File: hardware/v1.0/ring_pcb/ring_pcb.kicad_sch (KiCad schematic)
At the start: 18 parts

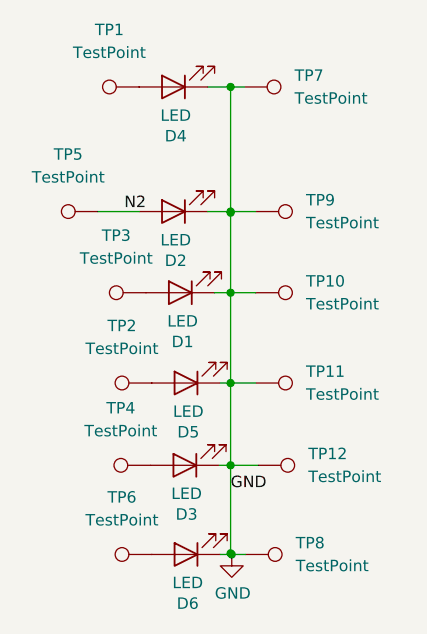
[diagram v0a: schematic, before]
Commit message: New PCB and Gerbers
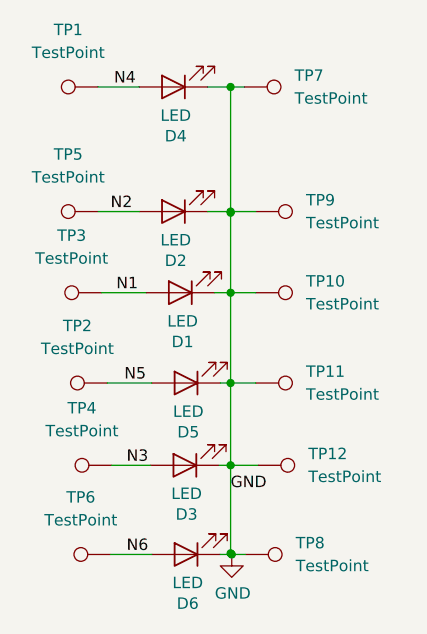
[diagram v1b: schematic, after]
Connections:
- net N4: now reaches D4.2 (A), TP1.1
- net N5: now reaches D5.2 (A), TP2.1
- net N3: now reaches D3.2 (A), TP4.1
- net N6: now reaches D6.2 (A), TP6.1
- net N1: now reaches D1.2 (A), TP3.1
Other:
- moved on the sheet: TP1, TP2, TP3, TP4, TP6
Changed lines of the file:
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@@
 (kicad_sch (version 20210621) (generator eeschema)
   (paper "A4")
+  (junction (at 127.508 87.757) (diameter 0) (color 0 0 0 0))
+  (junction (at 127.508 78.74) (diameter 0) (color 0 0 0 0))
   (junction (at 127.508 116.713) (diameter 0) (color 0 0 0 0))
-  (junction (at 127.508 87.757) (diameter 0) (color 0 0 0 0))
-  (junction (at 127.508 106.934) (diameter 0) (color 0 0 0 0))
-  (junction (at 127.508 78.74) (diameter 0) (color 0 0 0 0))
-  (junction (at 127.508 64.897) (diameter 0) (color 0 0 0 0))
   (junction (at 127.508 78.867) (diameter 0) (color 0 0 0 0))
   (junction (at 127.508 97.79) (diameter 0) (color 0 0 0 0))
+  (junction (at 127.508 64.897) (diameter 0) (color 0 0 0 0))
+  (junction (at 127.508 106.934) (diameter 0) (color 0 0 0 0))
   (junction (at 127.635 116.84) (diameter 0) (color 0 0 0 0))
+  (wire (pts (xy 113.792 97.79) (xy 118.745 97.79))
+    (stroke (width 0) (type default) (color 0 0 0 0))
+  )
   (wire (pts (xy 130.302 78.74) (xy 127.508 78.74))
     (stroke (width 0) (type default) (color 0 0 0 0))
@@
     (stroke (width 0) (type default) (color 0 0 0 0))
   )
+  (wire (pts (xy 114.173 116.84) (xy 118.745 116.84))
+    (stroke (width 0) (type default) (color 0 0 0 0))
+  )
   (wire (pts (xy 130.556 106.934) (xy 127.508 106.934))
     (stroke (width 0) (type default) (color 0 0 0 0))
   )
+  (wire (pts (xy 114.3 106.934) (xy 118.618 106.934))
+    (stroke (width 0) (type default) (color 0 0 0 0))
+  )
   (wire (pts (xy 112.776 78.74) (xy 117.348 78.74))
     (stroke (width 0) (type default) (color 0 0 0 0))
@@
     (stroke (width 0) (type default) (color 0 0 0 0))
   )
+  (wire (pts (xy 127.508 87.757) (xy 127.508 78.867))
+    (stroke (width 0) (type default) (color 0 0 0 0))
+  )
   (wire (pts (xy 127.508 78.867) (xy 127.508 78.74))
     (stroke (width 0) (type default) (color 0 0 0 0))
@@
     (stroke (width 0) (type default) (color 0 0 0 0))
   )
-  (wire (pts (xy 127.508 87.757) (xy 127.508 78.867))
+  (wire (pts (xy 127.508 97.79) (xy 127.508 87.757))
     (stroke (width 0) (type default) (color 0 0 0 0))
   )
@@
     (stroke (width 0) (type default) (color 0 0 0 0))
   )
-  (wire (pts (xy 127.508 97.79) (xy 127.508 87.757))
-    (stroke (width 0) (type default) (color 0 0 0 0))
-  )
   (wire (pts (xy 129.032 64.897) (xy 127.508 64.897))
     (stroke (width 0) (type default) (color 0 0 0 0))
@@
     (stroke (width 0) (type default) (color 0 0 0 0))
   )
+  (wire (pts (xy 112.776 64.897) (xy 117.348 64.897))
+    (stroke (width 0) (type default) (color 0 0 0 0))
+  )
+  (wire (pts (xy 129.159 116.84) (xy 127.635 116.84))
+    (stroke (width 0) (type default) (color 0 0 0 0))
+  )
   (wire (pts (xy 127.635 116.84) (xy 126.365 116.84))
     (stroke (width 0) (type default) (color 0 0 0 0))
   )
-  (wire (pts (xy 129.159 116.84) (xy 127.635 116.84))
-    (stroke (width 0) (type default) (color 0 0 0 0))
-  )
   (wire (pts (xy 126.238 106.934) (xy 127.508 106.934))
     (stroke (width 0) (type default) (color 0 0 0 0))
@@
     (stroke (width 0) (type default) (color 0 0 0 0))
   )
+  (wire (pts (xy 113.157 87.757) (xy 118.11 87.757))
+    (stroke (width 0) (type default) (color 0 0 0 0))
+  )
+  (label "N3" (at 115.951 106.934 0)
+    (effects (font (size 1.27 1.27)) (justify left bottom))
+  )
   (label "GND" (at 127.508 109.855 0)
     (effects (font (size 1.27 1.27)) (justify left bottom))
   )
-  (label "N2" (at 115.697 78.74 0)
+  (label "N1" (at 114.808 87.757 0)
+    (effects (font (size 1.27 1.27)) (justify left bottom))
+  )
+  (label "N5" (at 115.697 97.79 0)
+    (effects (font (size 1.27 1.27)) (justify left bottom))
+  )
+  (label "N2" (at 114.173 78.74 0)
+    (effects (font (size 1.27 1.27)) (justify left bottom))
+  )
+  (label "N4" (at 114.554 64.897 0)
+    (effects (font (size 1.27 1.27)) (justify left bottom))
+  )
+  (label "N6" (at 115.951 116.84 0)
     (effects (font (size 1.27 1.27)) (justify left bottom))
   )
@@
     (pin "2")
   )
-  (symbol (lib_id "Connector:TestPoint") (at 118.745 97.79 90) (unit 1)
-    (in_bom yes) (on_board yes) (fields_autoplaced)
-    (property "Reference" "TP2" (id 0) (at 115.443 91.44 90))
-    (property "Value" "TestPoint" (id 1) (at 115.443 93.98 90))
-    (property "Footprint" "TestPoint:TestPoint_Pad_1.5x1.5mm" (id 2) (at 118.745 92.71 0)
-      (effects (font (size 1.27 1.27)) hide)
-    )
-    (property "Datasheet" "~" (id 3) (at 118.745 92.71 0)
+  (symbol (lib_id "Connector:TestPoint") (at 113.792 97.79 90) (unit 1)
+    (in_bom yes) (on_board yes) (fields_autoplaced)
+    (property "Reference" "TP2" (id 0) (at 110.49 91.44 90))
+    (property "Value" "TestPoint" (id 1) (at 110.49 93.98 90))
+    (property "Footprint" "TestPoint:TestPoint_Pad_1.5x1.5mm" (id 2) (at 113.792 92.71 0)
+      (effects (font (size 1.27 1.27)) hide)
+    )
+    (property "Datasheet" "~" (id 3) (at 113.792 92.71 0)
       (effects (font (size 1.27 1.27)) hide)
     )
@@
     (pin "1")
   )
-  (symbol (lib_id "Connector:TestPoint") (at 118.745 116.84 90) (unit 1)
-    (in_bom yes) (on_board yes) (fields_autoplaced)
-    (property "Reference" "TP6" (id 0) (at 115.443 110.49 90))
-    (property "Value" "TestPoint" (id 1) (at 115.443 113.03 90))
-    (property "Footprint" "TestPoint:TestPoint_Pad_1.5x1.5mm" (id 2) (at 118.745 111.76 0)
-      (effects (font (size 1.27 1.27)) hide)
-    )
-    (property "Datasheet" "~" (id 3) (at 118.745 111.76 0)
+  (symbol (lib_id "Connector:TestPoint") (at 114.173 116.84 90) (unit 1)
+    (in_bom yes) (on_board yes) (fields_autoplaced)
+    (property "Reference" "TP6" (id 0) (at 110.871 110.49 90))
+    (property "Value" "TestPoint" (id 1) (at 110.871 113.03 90))
+    (property "Footprint" "TestPoint:TestPoint_Pad_1.5x1.5mm" (id 2) (at 114.173 111.76 0)
+      (effects (font (size 1.27 1.27)) hide)
+    )
+    (property "Datasheet" "~" (id 3) (at 114.173 111.76 0)
       (effects (font (size 1.27 1.27)) hide)
     )
@@
     (pin "1")
   )
-  (symbol (lib_id "Connector:TestPoint") (at 118.11 87.757 90) (unit 1)
-    (in_bom yes) (on_board yes) (fields_autoplaced)
-    (property "Reference" "TP3" (id 0) (at 114.808 81.407 90))
-    (property "Value" "TestPoint" (id 1) (at 114.808 83.947 90))
-    (property "Footprint" "TestPoint:TestPoint_Pad_1.5x1.5mm" (id 2) (at 118.11 82.677 0)
-      (effects (font (size 1.27 1.27)) hide)
-    )
-    (property "Datasheet" "~" (id 3) (at 118.11 82.677 0)
-      (effects (font (size 1.27 1.27)) hide)
-    )
-    (pin "1")
-  )
-  (symbol (lib_id "Connector:TestPoint") (at 117.348 64.897 90) (unit 1)
-    (in_bom yes) (on_board yes) (fields_autoplaced)
-    (property "Reference" "TP1" (id 0) (at 114.046 58.547 90))
-    (property "Value" "TestPoint" (id 1) (at 114.046 61.087 90))
-    (property "Footprint" "TestPoint:TestPoint_Pad_1.5x1.5mm" (id 2) (at 117.348 59.817 0)
-      (effects (font (size 1.27 1.27)) hide)
-    )
-    (property "Datasheet" "~" (id 3) (at 117.348 59.817 0)
-      (effects (font (size 1.27 1.27)) hide)
-    )
-    (pin "1")
-  )
-  (symbol (lib_id "Connector:TestPoint") (at 118.618 106.934 90) (unit 1)
-    (in_bom yes) (on_board yes) (fields_autoplaced)
-    (property "Reference" "TP4" (id 0) (at 115.316 100.584 90))
-    (property "Value" "TestPoint" (id 1) (at 115.316 103.124 90))
-    (property "Footprint" "TestPoint:TestPoint_Pad_1.5x1.5mm" (id 2) (at 118.618 101.854 0)
-      (effects (font (size 1.27 1.27)) hide)
-    )
-    (property "Datasheet" "~" (id 3) (at 118.618 101.854 0)
-      (effects (font (size 1.27 1.27)) hide)
-    )
+  (symbol (lib_id "Connector:TestPoint") (at 113.157 87.757 90) (unit 1)
+    (in_bom yes) (on_board yes) (fields_autoplaced)
+    (property "Reference" "TP3" (id 0) (at 109.855 81.407 90))
+    (property "Value" "TestPoint" (id 1) (at 109.855 83.947 90))
+    (property "Footprint" "TestPoint:TestPoint_Pad_1.5x1.5mm" (id 2) (at 113.157 82.677 0)
+      (effects (font (size 1.27 1.27)) hide)
+    )
+    (property "Datasheet" "~" (id 3) (at 113.157 82.677 0)
+      (effects (font (size 1.27 1.27)) hide)
+    )
+    (pin "1")
+  )
+  (symbol (lib_id "Connector:TestPoint") (at 112.776 64.897 90) (unit 1)
+    (in_bom yes) (on_board yes) (fields_autoplaced)
+    (property "Reference" "TP1" (id 0) (at 109.474 58.547 90))
+    (property "Value" "TestPoint" (id 1) (at 109.474 61.087 90))
+    (property "Footprint" "TestPoint:TestPoint_Pad_1.5x1.5mm" (id 2) (at 112.776 59.817 0)
+      (effects (font (size 1.27 1.27)) hide)
+    )
+    (property "Datasheet" "~" (id 3) (at 112.776 59.817 0)
+      (effects (font (size 1.27 1.27)) hide)
+    )
+    (pin "1")
+  )
+  (symbol (lib_id "Connector:TestPoint") (at 114.3 106.934 90) (unit 1)
+    (in_bom yes) (on_board yes) (fields_autoplaced)
+    (property "Reference" "TP4" (id 0) (at 110.998 100.584 90))
+    (property "Value" "TestPoint" (id 1) (at 110.998 103.124 90))
+    (property "Footprint" "TestPoint:TestPoint_Pad_1.5x1.5mm" (id 2) (at 114.3 101.854 0)
+      (effects (font (size 1.27 1.27)) hide)
+    )
+    (property "Datasheet" "~" (id 3) (at 114.3 101.854 0)
+      (effects (font (size 1.27 1.27)) hide)
+    )
